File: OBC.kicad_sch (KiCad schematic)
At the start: 11 parts, among them J1 I2C, J2 Conn_02x07_Counter_Clockwise, J6 SWD, J7 RMF, SW3 SW_Push, SW5 RST, U1 E73-2G4M08S1C, Y1 32.768

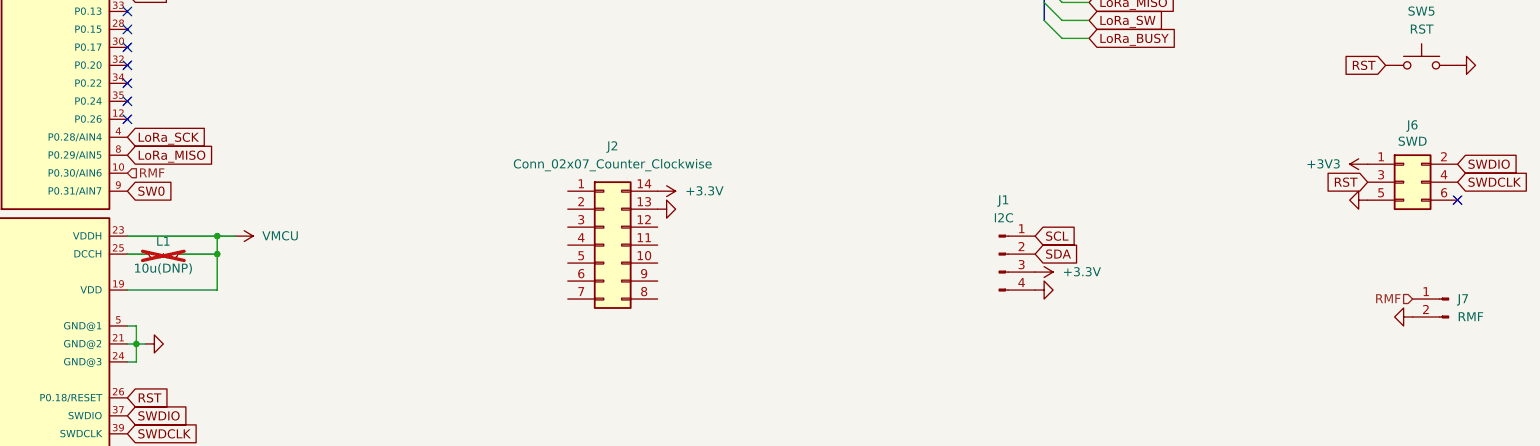
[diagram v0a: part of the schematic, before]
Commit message: Started PCB layout
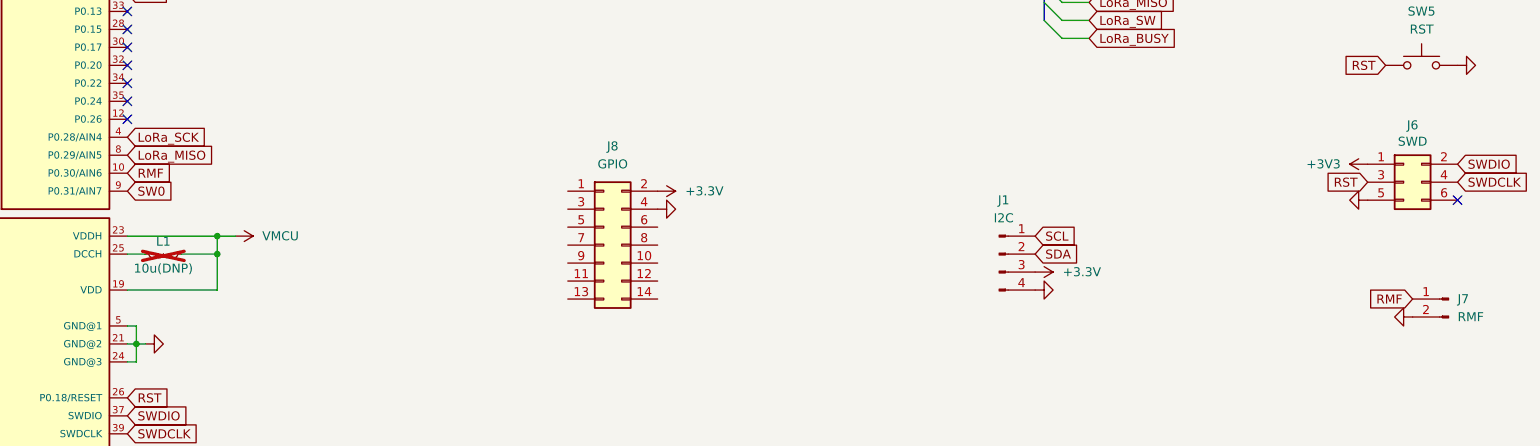
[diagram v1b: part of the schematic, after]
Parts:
- removed J2: Conn_02x07_Counter_Clockwise, symbol Connector_Generic:Conn_02x07_Counter_Clockwise
- added J8: GPIO, Connector_PinHeader_2.54mm:PinHeader_2x07_P2.54mm_Vertical, symbol Connector_Generic:Conn_02x07_Odd_Even
- J1: footprint (none) -> Connector_PinHeader_2.54mm:PinHeader_1x04_P2.54mm_Vertical
- L1: footprint Inductor_SMD:L_Changjiang_FTC201610D -> Inductor_SMD:L_1210_3225Metric
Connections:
- net +3.3V: now also J8.2 (Pin_2)
- net GND: now also J8.4 (Pin_4)
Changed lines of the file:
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@@
+		)
+	)
+	(global_label "RMF"
+		(shape input)
+		(at 68.58 115.57 0)
+		(fields_autoplaced yes)
+		(effects
+			(font
+				(size 1.27 1.27)
+			)
+			(justify left)
+		)
+		(property "Intersheetrefs" "${INTERSHEET_REFS}"
+			(at 75.3752 115.57 0)
+			(hide yes)
+			(show_name no)
+			(do_not_autoplace no)
+			(effects
+				(font
+					(size 1.27 1.27)
+				)
+				(justify left)
+			)
 		)
 	)
@@
 		)
 	)
+	(global_label "RMF"
+		(shape input)
+		(at 250.19 133.35 180)
+		(fields_autoplaced yes)
+		(effects
+			(font
+				(size 1.27 1.27)
+			)
+			(justify right)
+		)
+		(property "Intersheetrefs" "${INTERSHEET_REFS}"
+			(at 243.3948 133.35 0)
+			(hide yes)
+			(show_name no)
+			(do_not_autoplace no)
+			(effects
+				(font
+					(size 1.27 1.27)
+				)
+				(justify right)
+			)
+		)
+	)
 	(global_label "LoRa_SCK"
 		(shape input)
@@
 		)
 	)
-	(hierarchical_label "RMF"
-		(shape input)
-		(at 68.58 115.57 0)
-		(effects
-			(font
-				(size 1.27 1.27)
-			)
-			(justify left)
-		)
-	)
 	(hierarchical_label "{LoRa_BUS}"
 		(shape input)
@@
 			)
 			(justify left)
-		)
-	)
-	(hierarchical_label "RMF"
-		(shape input)
-		(at 250.19 133.35 180)
-		(effects
-			(font
-				(size 1.27 1.27)
-			)
-			(justify right)
 		)
 	)
@@
 	)
 	(symbol
+		(lib_id "Connector_Generic:Conn_02x07_Odd_Even")
+		(at 135.89 125.73 0)
+		(unit 1)
+		(body_style 1)
+		(exclude_from_sim no)
+		(in_bom yes)
+		(on_board yes)
+		(in_pos_files yes)
+		(dnp no)
+		(fields_autoplaced yes)
+		(property "Reference" "J8"
+			(at 137.16 111.76 0)
+			(show_name no)
+			(do_not_autoplace no)
+			(effects
+				(font
+					(size 1.27 1.27)
+				)
+			)
+		)
+		(property "Value" "GPIO"
+			(at 137.16 114.3 0)
+			(show_name no)
+			(do_not_autoplace no)
+			(effects
+				(font
+					(size 1.27 1.27)
+				)
+			)
+		)
+		(property "Footprint" "Connector_PinHeader_2.54mm:PinHeader_2x07_P2.54mm_Vertical"
+			(at 135.89 125.73 0)
+			(hide yes)
+			(show_name no)
+			(do_not_autoplace no)
+			(effects
+				(font
+					(size 1.27 1.27)
+				)
+			)
+		)
+		(property "Datasheet" ""
+			(at 135.89 125.73 0)
+			(hide yes)
+			(show_name no)
+			(do_not_autoplace no)
+			(effects
+				(font
+					(size 1.27 1.27)
+				)
+			)
+		)
+		(property "Description" "Generic connector, double row, 02x07, odd/even pin numbering scheme (row 1 odd numbers, row 2 even numbers), script generated (kicad-library-utils/schlib/autogen/connector/)"
+			(at 135.89 125.73 0)
+			(hide yes)
+			(show_name no)
+			(do_not_autoplace no)
+			(effects
+				(font
+					(size 1.27 1.27)
+				)
+			)
+		)
+		(pin "14"
+		)
+		(pin "13"
+		)
+		(pin "12"
+		)
+		(pin "11"
+		)
+		(pin "10"
+		)
+		(pin "1"
+		)
+		(pin "3"
+		)
+		(pin "2"
+		)
+		(pin "4"
+		)
+		(pin "6"
+		)
+		(pin "7"
+		)
+		(pin "5"
+		)
+		(pin "9"
+		)
+		(pin "8"
+		)
+		(instances
+			(project "CanSat_Devboard"
+				(path "/f9e05184-c88b-4a88-ae9c-ab2bdb32be7c/5d00bd0a-3bbf-46b2-b8c5-f75441fb4350/2028456c-6ef4-4d71-987d-d023cb9d3da5"
+					(reference "J8")
+					(unit 1)
+				)
+			)
+		)
+	)
+	(symbol
 		(lib_id "power:GND")
 		(at 256.54 100.33 90)
@@
 			)
 		)
-		(property "Footprint" "Inductor_SMD:L_Changjiang_FTC201610D"
+		(property "Footprint" "Inductor_SMD:L_1210_3225Metric"
 			(at 73.66 127 0)
 			(hide yes)
@@
 			)
 		)
-		(property "Footprint" ""
+		(property "Footprint" "Connector_PinHeader_2.54mm:PinHeader_1x04_P2.54mm_Vertical"
 			(at 191.77 127 0)
 			(hide yes)
@@
 					(unit 1)
 				)
-			)
-		)
-	)
-	(symbol
-		(lib_id "Connector_Generic:Conn_02x07_Counter_Clockwise")
-		(at 135.89 125.73 0)
-		(unit 1)
-		(body_style 1)
-		(exclude_from_sim no)
-		(in_bom yes)
-		(on_board yes)
-		(in_pos_files yes)
-		(dnp no)
-		(fields_autoplaced yes)
-		(property "Reference" "J2"
-			(at 137.16 111.76 0)
-			(show_name no)
-			(do_not_autoplace no)
-			(effects
-				(font
-					(size 1.27 1.27)
-				)
-			)
-		)
-		(property "Value" "Conn_02x07_Counter_Clockwise"
-			(at 137.16 114.3 0)
-			(show_name no)
-			(do_not_autoplace no)
-			(effects
-				(font
-					(size 1.27 1.27)
-				)
-			)
-		)
-		(property "Footprint" ""
-			(at 135.89 125.73 0)
-			(hide yes)
-			(show_name no)
-			(do_not_autoplace no)
-			(effects
-				(font
-					(size 1.27 1.27)
-				)
-			)
-		)
-		(property "Datasheet" ""
-			(at 135.89 125.73 0)
-			(hide yes)
-			(show_name no)
-			(do_not_autoplace no)
-			(effects
-				(font
-					(size 1.27 1.27)
-				)
-			)
-		)
-		(property "Description" "Generic connector, double row, 02x07, counter clockwise pin numbering scheme (similar to DIP package numbering), script generated (kicad-library-utils/schlib/autogen/connector/)"
-			(at 135.89 125.73 0)
-			(hide yes)
-			(show_name no)
-			(do_not_autoplace no)
-			(effects
-				(font
-					(size 1.27 1.27)
-				)
-			)
-		)
-		(pin "1"
-		)
-		(pin "12"
-		)
-		(pin "2"
-		)
-		(pin "6"
-		)
-		(pin "7"
-		)
-		(pin "14"
-		)
-		(pin "3"
-		)
-		(pin "8"
-		)
-		(pin "9"
-		)
-		(pin "5"
-		)
-		(pin "13"
-		)
-		(pin "11"
-		)
-		(pin "4"
-		)
-		(pin "10"
-		)
-		(instances
-			(project "CanSat_Devboard"
-				(path "/f9e05184-c88b-4a88-ae9c-ab2bdb32be7c/5d00bd0a-3bbf-46b2-b8c5-f75441fb4350/2028456c-6ef4-4d71-987d-d023cb9d3da5"
-					(reference "J2")
-					(unit 1)
-				)
